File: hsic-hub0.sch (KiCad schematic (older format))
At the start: 17 parts

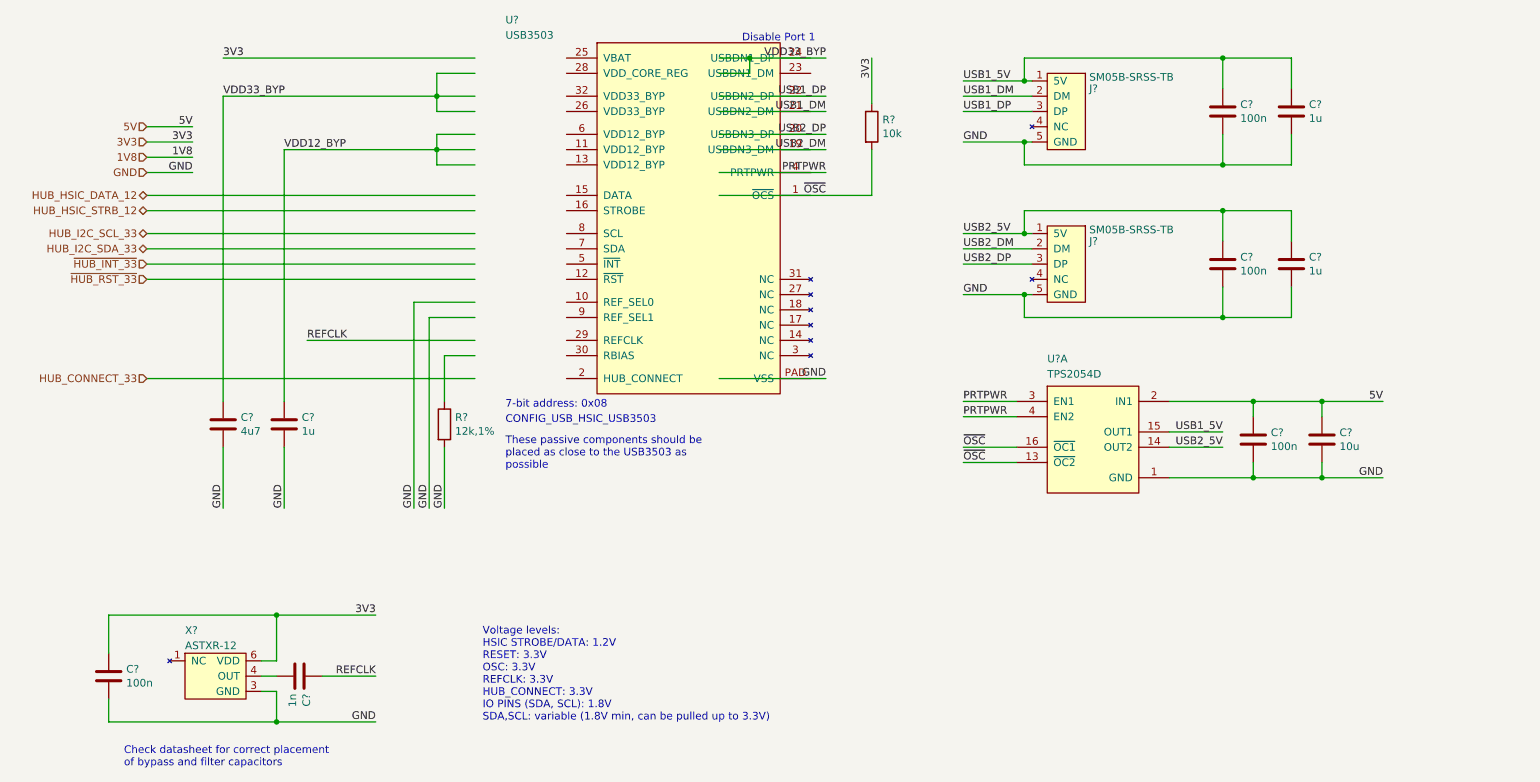
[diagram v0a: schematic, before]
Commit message: Minor fixes.
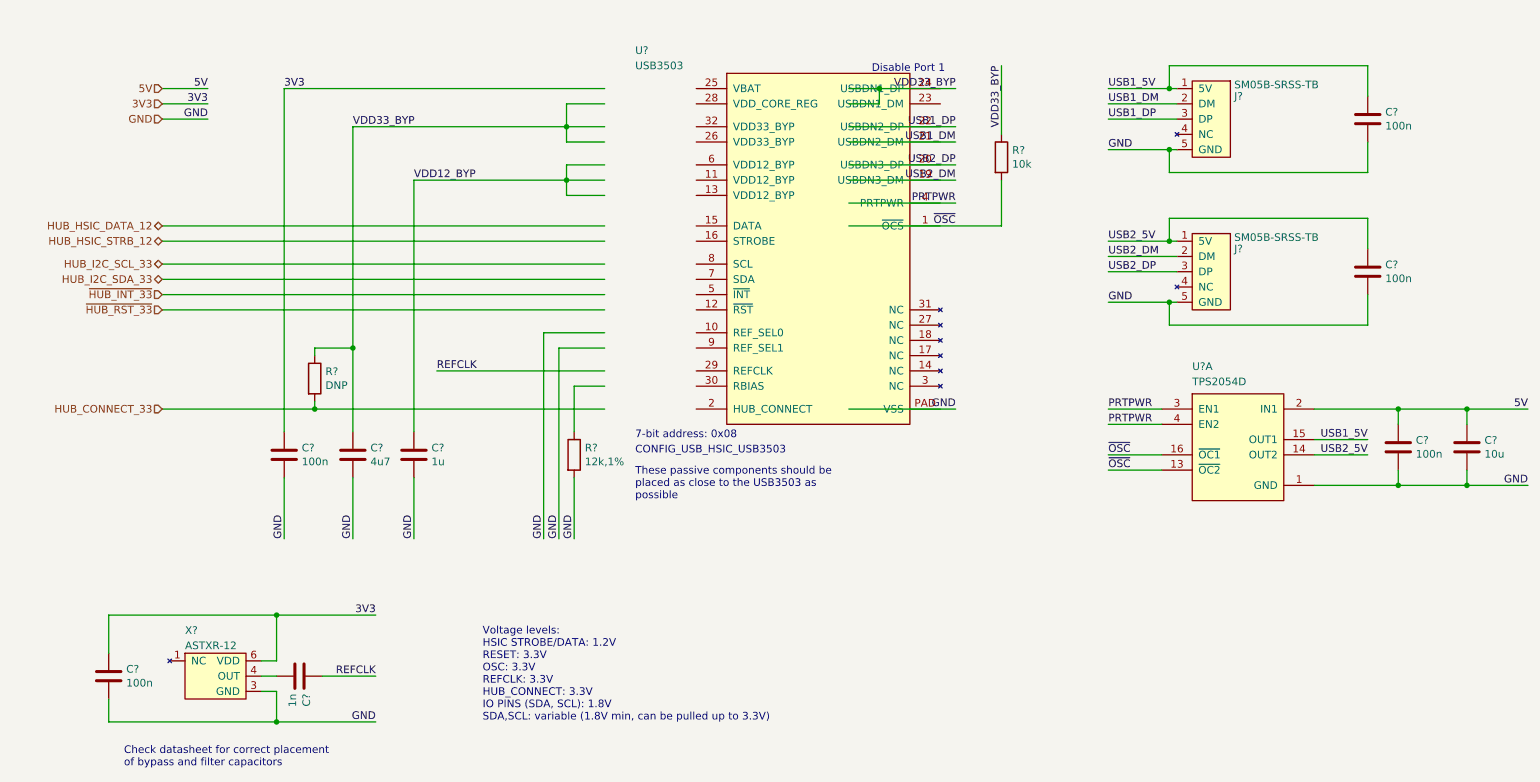
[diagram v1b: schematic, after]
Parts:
- removed C? (x2): 1u, Capacitor_SMD:C_0805_2012Metric_Pad1.15x1.40mm_HandSolder, symbol Drone:CAP
- added C?: 100n, Capacitor_SMD:C_0805_2012Metric_Pad1.15x1.40mm_HandSolder, symbol Drone:CAP
- added R?: DNP, Resistor_SMD:R_0805_2012Metric_Pad1.15x1.40mm_HandSolder, symbol Drone:RES
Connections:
- net labels removed: 1V8
- wire segments 109 -> 107
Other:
- moved on the sheet: C?, J?, R?, U?, U?A
